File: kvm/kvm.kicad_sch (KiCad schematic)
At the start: 61 parts, among them J1 USB_C_Receptacle_USB2.0, J2 USB_C_Receptacle_USB2.0, J3 USB_A_Stacked, J4 USB_A_Stacked, Q1 Q_PMOS_GSD, SW1 SW_DPDT_x2, U1 FSUSB42MUX, U2 LTC4412xS6, U3 GL850G, U4 SRV05-4, U5 SRV05-4, U6 SRV05-4, Y1 Crystal

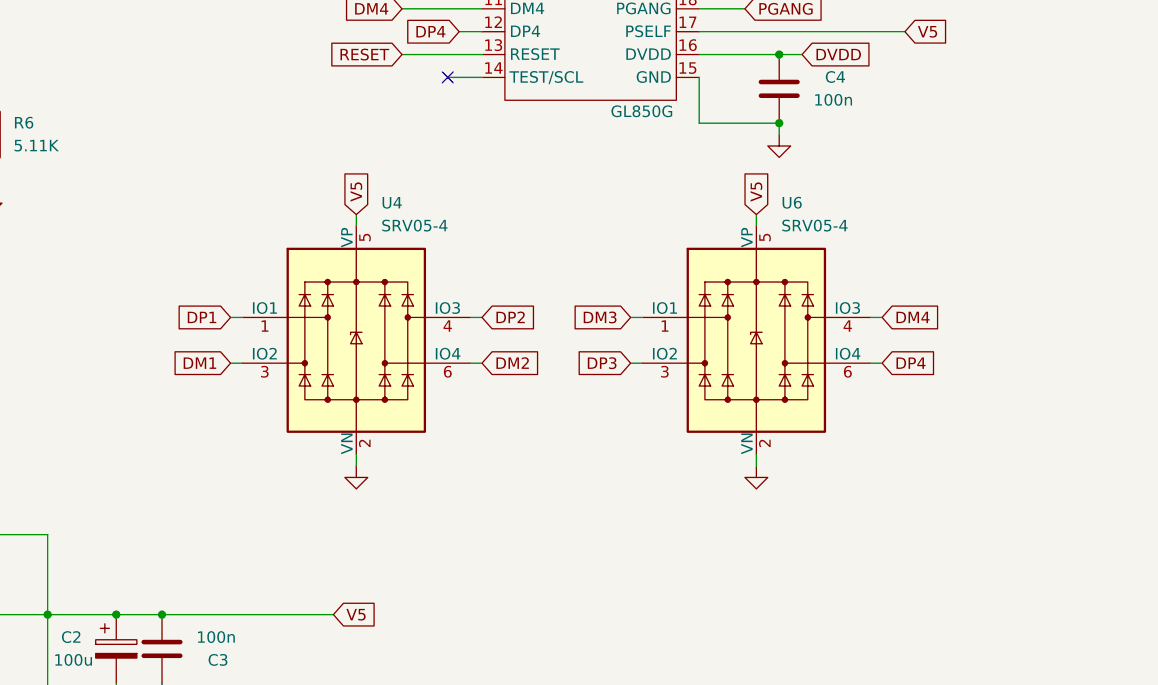
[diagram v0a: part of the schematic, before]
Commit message: first layout version
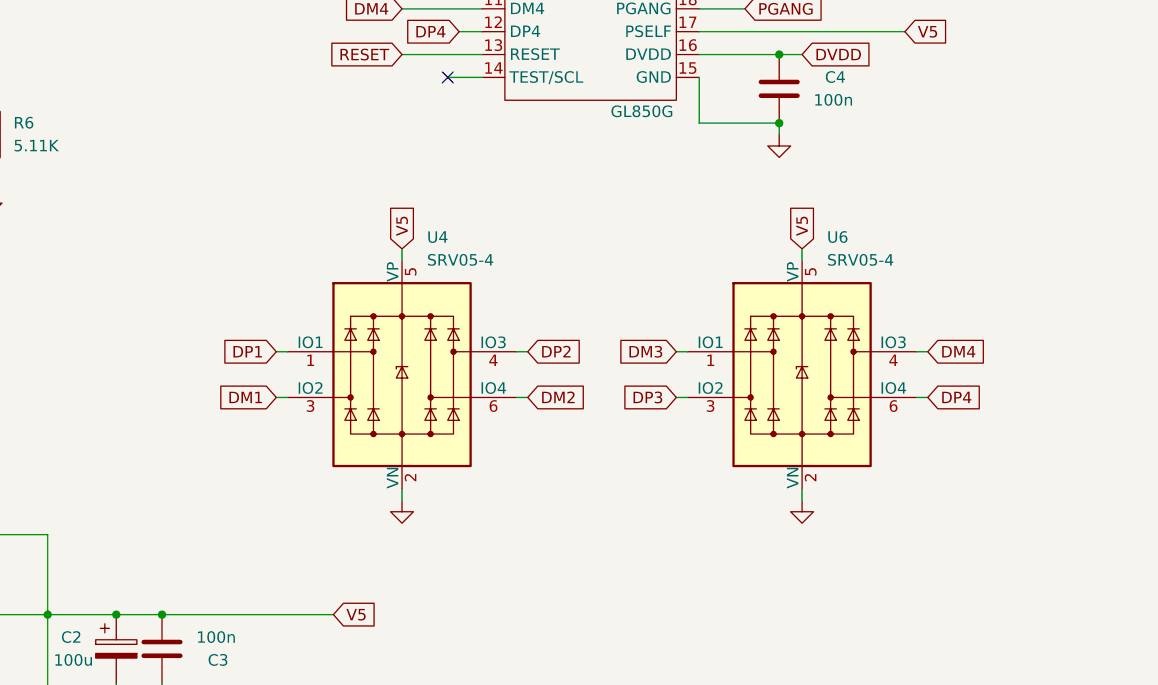
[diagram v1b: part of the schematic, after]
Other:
- moved on the sheet: U4, U6
